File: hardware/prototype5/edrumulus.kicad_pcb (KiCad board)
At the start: 2 copper layers, 65 x 56.5 mm, 67 parts, among them J1 Trigger Connector, J2 Raspberry Pi GPIO pins, U1 ESP32-DEVKIT-V1

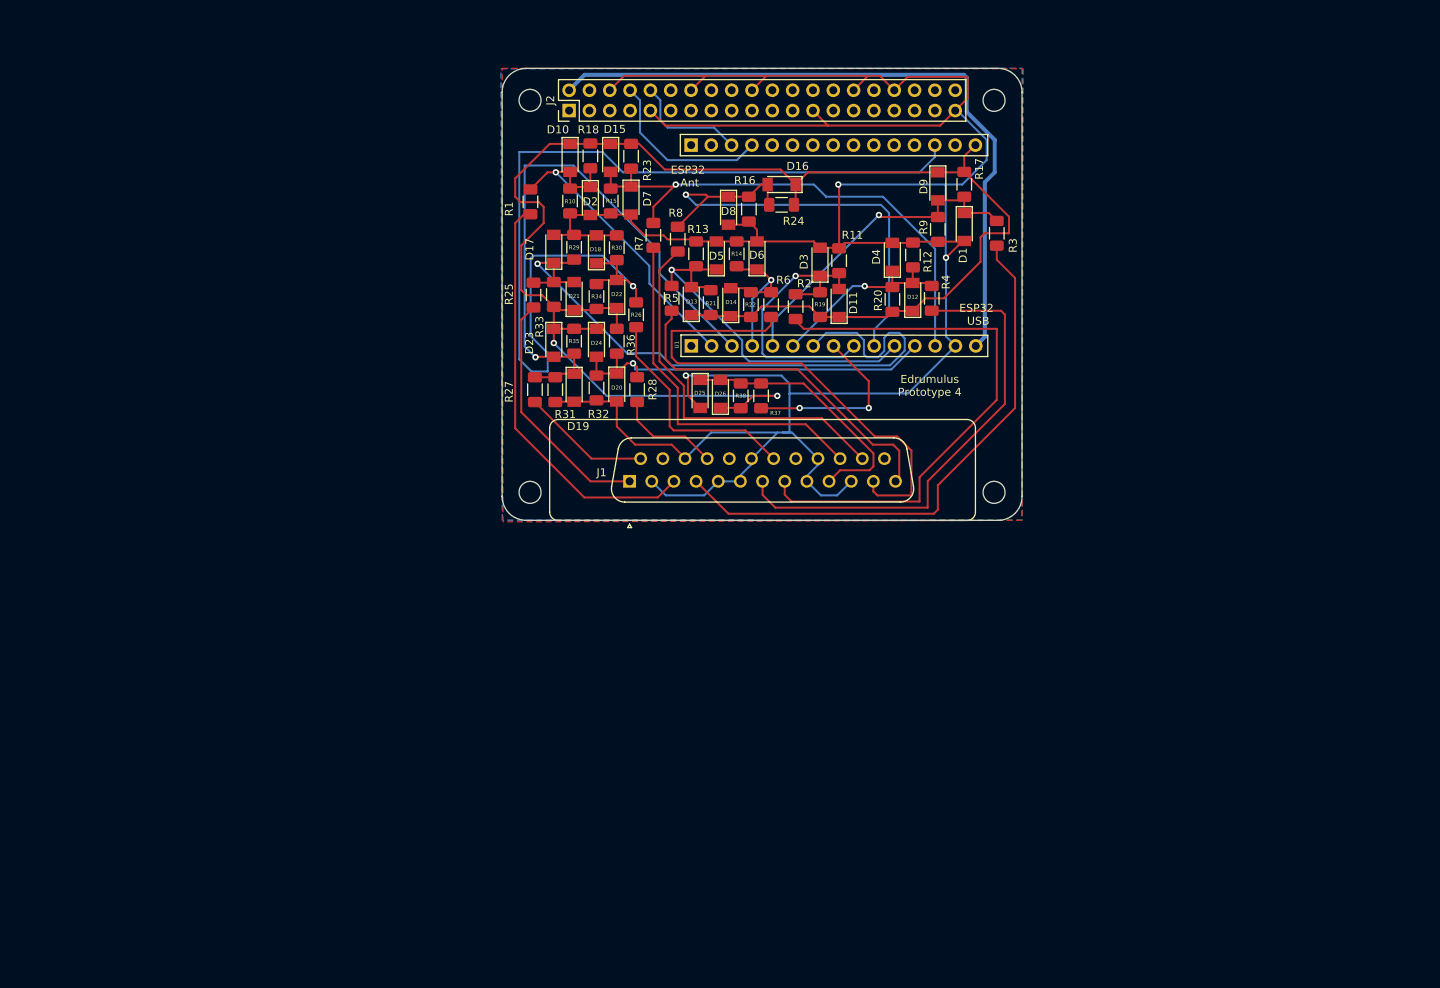
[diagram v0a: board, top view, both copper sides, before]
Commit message: some layout cleanup
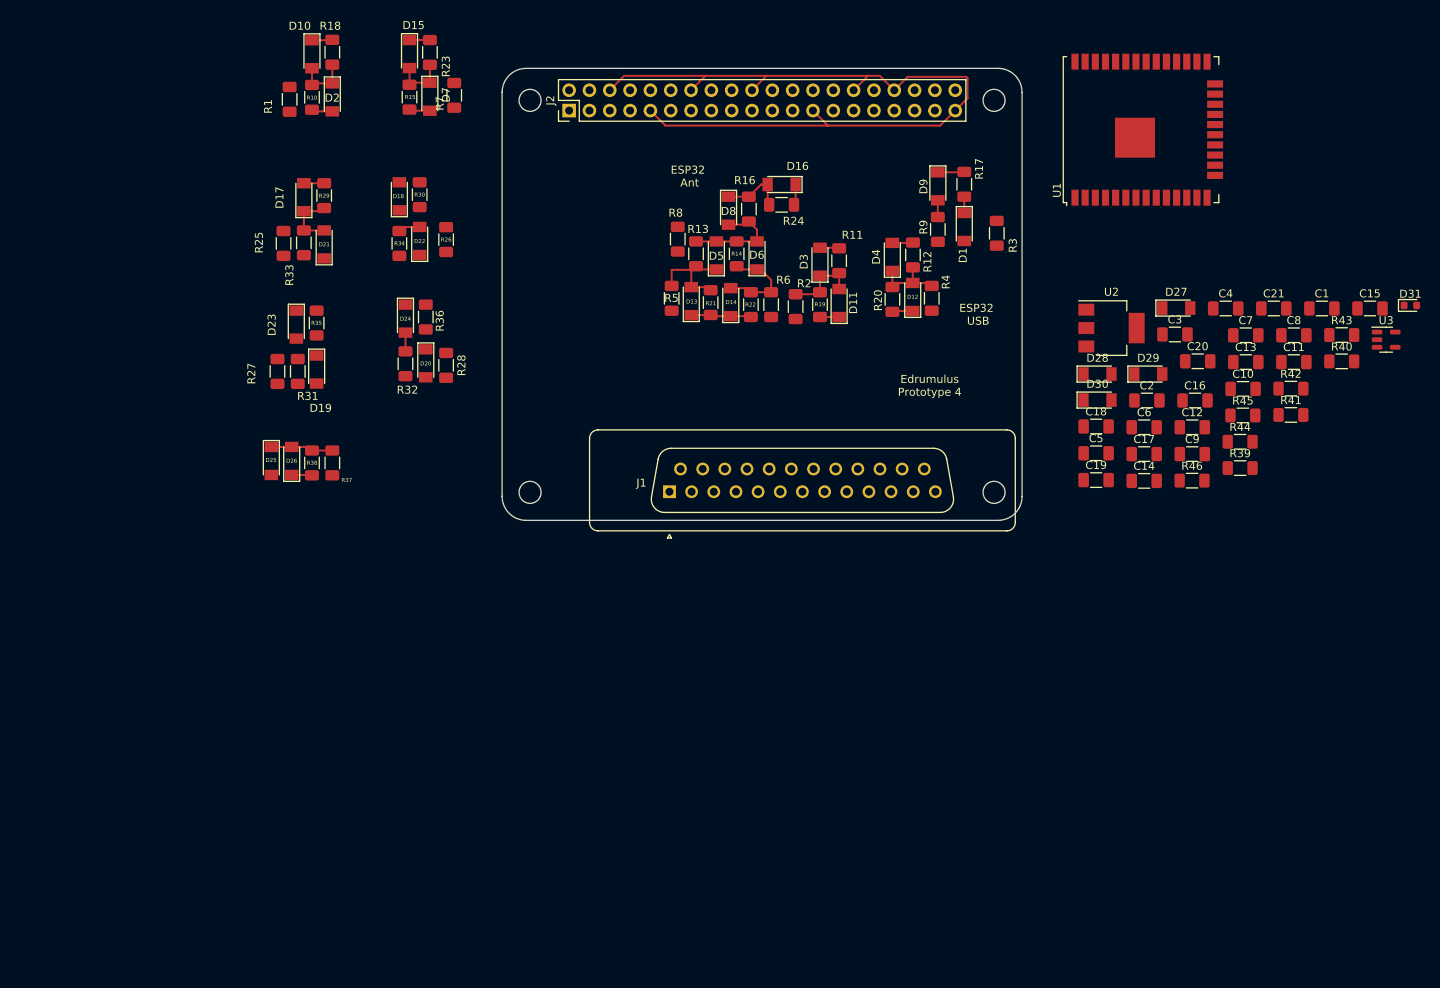
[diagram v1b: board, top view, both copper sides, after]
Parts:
- added C1: 100 nF, Capacitor_SMD:C_1206_3216Metric_Pad1.33x1.80mm_HandSolder, F.Cu at (209.0, 103.1)
- added C10: 100 nF, Capacitor_SMD:C_1206_3216Metric_Pad1.33x1.80mm_HandSolder, F.Cu at (199.2, 113.2)
- added C11: 100 nF, Capacitor_SMD:C_1206_3216Metric_Pad1.33x1.80mm_HandSolder, F.Cu at (205.5, 109.8)
- added C12: 100 nF, Capacitor_SMD:C_1206_3216Metric_Pad1.33x1.80mm_HandSolder, F.Cu at (192.8, 118.0)
- added C13: 100 nF, Capacitor_SMD:C_1206_3216Metric_Pad1.33x1.80mm_HandSolder, F.Cu at (199.5, 109.8)
- added C14: 100 nF, Capacitor_SMD:C_1206_3216Metric_Pad1.33x1.80mm_HandSolder, F.Cu at (186.8, 124.7)
- added C15: 100 nF, Capacitor_SMD:C_1206_3216Metric_Pad1.33x1.80mm_HandSolder, F.Cu at (215.1, 103.1)
- added C16: 1 µF, Capacitor_SMD:C_1206_3216Metric_Pad1.33x1.80mm_HandSolder, F.Cu at (193.2, 114.6)
- added C17: 22 µF, Capacitor_SMD:C_1206_3216Metric_Pad1.33x1.80mm_HandSolder, F.Cu at (186.8, 121.3)
- added C18: 10 nF, Capacitor_SMD:C_1206_3216Metric_Pad1.33x1.80mm_HandSolder, F.Cu at (180.8, 117.9)
- added C19: 10 µF, Capacitor_SMD:C_1206_3216Metric_Pad1.33x1.80mm_HandSolder, F.Cu at (180.8, 124.6)
- added C2: 100 nF, Capacitor_SMD:C_1206_3216Metric_Pad1.33x1.80mm_HandSolder, F.Cu at (187.2, 114.6)
- added C20: 1 µF, Capacitor_SMD:C_1206_3216Metric_Pad1.33x1.80mm_HandSolder, F.Cu at (193.5, 109.7)
- added C21: 22 µF, Capacitor_SMD:C_1206_3216Metric_Pad1.33x1.80mm_HandSolder, F.Cu at (203.0, 103.1)
- added C3: 100 nF, Capacitor_SMD:C_1206_3216Metric_Pad1.33x1.80mm_HandSolder, F.Cu at (190.7, 106.4)
- added C4: 100 nF, Capacitor_SMD:C_1206_3216Metric_Pad1.33x1.80mm_HandSolder, F.Cu at (197.0, 103.1)
- added C5: 100 nF, Capacitor_SMD:C_1206_3216Metric_Pad1.33x1.80mm_HandSolder, F.Cu at (180.8, 121.2)
- added C6: 100 nF, Capacitor_SMD:C_1206_3216Metric_Pad1.33x1.80mm_HandSolder, F.Cu at (186.8, 118.0)
- added C7: 100 nF, Capacitor_SMD:C_1206_3216Metric_Pad1.33x1.80mm_HandSolder, F.Cu at (199.5, 106.5)
- added C8: 100 nF, Capacitor_SMD:C_1206_3216Metric_Pad1.33x1.80mm_HandSolder, F.Cu at (205.5, 106.5)
- added C9: 100 nF, Capacitor_SMD:C_1206_3216Metric_Pad1.33x1.80mm_HandSolder, F.Cu at (192.8, 121.3)
- added D27: BAT85, Diode_SMD:D_MiniMELF, F.Cu at (190.8, 103.1)
- added D28: BAT85, Diode_SMD:D_MiniMELF, F.Cu at (181.0, 111.3)
- added D29: BAT85, Diode_SMD:D_MiniMELF, F.Cu at (187.3, 111.3)
- added D30: BAT85, Diode_SMD:D_MiniMELF, F.Cu at (181.0, 114.6)
- added D31: BOARD-LED, LED_SMD:LED_0603_1608Metric, F.Cu at (220.1, 102.7)
- added R39: 22 kOhm, Resistor_SMD:R_1206_3216Metric_Pad1.30x1.75mm_HandSolder, F.Cu at (198.8, 123.1)
- added R40: 22 kOhm, Resistor_SMD:R_1206_3216Metric_Pad1.30x1.75mm_HandSolder, F.Cu at (211.5, 109.7)
- added R41: 22 kOhm, Resistor_SMD:R_1206_3216Metric_Pad1.30x1.75mm_HandSolder, F.Cu at (205.2, 116.4)
- added R42: 22 kOhm, Resistor_SMD:R_1206_3216Metric_Pad1.30x1.75mm_HandSolder, F.Cu at (205.2, 113.1)
- added R43: 22 kOhm, Resistor_SMD:R_1206_3216Metric_Pad1.30x1.75mm_HandSolder, F.Cu at (211.5, 106.4)
- added R44: 22 kOhm, Resistor_SMD:R_1206_3216Metric_Pad1.30x1.75mm_HandSolder, F.Cu at (198.8, 119.8)
- added R45: 10 kOhm, Resistor_SMD:R_1206_3216Metric_Pad1.30x1.75mm_HandSolder, F.Cu at (199.2, 116.5)
- added R46: 470 Ohm, Resistor_SMD:R_1206_3216Metric_Pad1.30x1.75mm_HandSolder, F.Cu at (192.8, 124.6)
- added U2: AMS1117-3.3, Package_TO_SOT_SMD:SOT-223-3_TabPin2, F.Cu at (182.7, 105.6)
- added U3: LT1761-3.3, Package_TO_SOT_SMD:TSOT-23-5, F.Cu at (217.1, 107.0)
- R27, R28: value 100 kOhm -> 22 kOhm
- R30, R32, R35, R36: value 22 kOhm -> 100 kOhm
- U1: value ESP32-DEVKIT-V1 -> ESP32-WROOM-32U; footprint edrumulus:esp32_devkit_v1 -> RF_Module:ESP32-WROOM-32U
- moved U1 62.4 mm to (186.4, 80.8)
- moved D25 54.2 mm to (77.7, 122.2)
- moved D26 54.2 mm to (80.3, 122.2)
- moved R37 54.2 mm to (85.3, 122.4)
- moved R38 54.2 mm to (82.8, 122.4)
- moved R18 34.8 mm to (85.3, 71.1)
- moved D2 34.8 mm to (85.3, 76.7)
- moved R10 34.8 mm to (82.8, 76.7)
- moved D10 34.8 mm to (82.8, 71.3)
- moved R1 32.7 mm to (80.0, 77.0)
- moved D19 32.3 mm to (83.4, 110.8)
- moved D23 32.3 mm to (80.8, 105.1)
- moved R27 32.3 mm to (78.5, 111.0)
- moved R31 32.3 mm to (81.0, 111.0)
- moved R35 32.3 mm to (83.4, 104.9)
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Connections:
- D18 pad 1: GPIO15 -> GPIO2
- D19 pad 1: GPIO39 -> 3V3
- D19 pad 2: CRASH1-SLEEVE -> GPIO2
- D22 pad 1: 3V3 -> GPIO15
- D22 pad 2: GPIO15 -> CRASH1-SLEEVE
- D23 pad 2: GPIO39 -> GPIO12
- D24 pad 2: GPIO12 -> GPIO15
- J1 pad 15: unconnected-(J1-Pad15) -> TOM1-RING
- J1 pad 25: unconnected-(J1-Pad25) -> RIDE-BELL-TIP
- J2 pad 2: ESP-VIN -> RASPI-VIN
- R25 pad 1: KICK-TIP -> GPIO33
- R25 pad 2: GPIO33 -> KICK-TIP
- R26 pad 1: TOM3-TIP -> RIDE-BELL-TIP
- R26 pad 2: GPIO15 -> GPIO2
- R27 pad 1: TOM1-TIP -> GPIO2
- R27 pad 2: GPIO39 -> CRASH1-SLEEVE
- R28 pad 1: TOM2-TIP -> 3V3
- R28 pad 2: GPIO12 -> GPIO2
- R30 pad 1: GPIO15 -> GPIO12
- R30 pad 2: CRASH1-SLEEVE -> TOM2-TIP
- R31 pad 1: GPIO39 -> GPIO12
- R32 pad 1: GPIO12 -> GPIO15
- R32 pad 2: CRASH1-SLEEVE -> TOM3-TIP
- R34 pad 1: 3V3 -> GPIO15
- R34 pad 2: GPIO15 -> CRASH1-SLEEVE
- R35 pad 1: 3V3 -> TOM1-RING
- R35 pad 2: GPIO39 -> GPIO4
- R36 pad 1: 3V3 -> TOM1-TIP
- R36 pad 2: GPIO12 -> GPIO39
- U1 pad 1: unconnected-(U1-Pad1) -> CRASH1-SLEEVE
- U1 pad 10: GPIO27 -> GPIO25
- U1 pad 11: GPIO14 -> GPIO26
- U1 pad 12: GPIO12 -> GPIO27
- U1 pad 13: GPIO13 -> GPIO14
- U1 pad 14: CRASH1-SLEEVE -> GPIO12
- U1 pad 15: ESP-VIN -> CRASH1-SLEEVE
- U1 pad 16: 3V3 -> GPIO13
- U1 pad 17: CRASH1-SLEEVE -> unconnected-(U1-Pad17)
- U1 pad 18: GPIO15 -> unconnected-(U1-Pad18)
- U1 pad 2: GPIO36 -> ESP32-3V3
- U1 pad 23: unconnected-(U1-Pad23) -> GPIO15
- U1 pad 24: unconnected-(U1-Pad24) -> GPIO2
- U1 pad 26: unconnected-(U1-Pad26) -> GPIO4
- U1 pad 27: ESP-UART0-RX -> unconnected-(U1-Pad27)
- U1 pad 28: ESP-UART0-TX -> unconnected-(U1-Pad28)
- U1 pad 29: unconnected-(U1-Pad29) -> Net-(R46-Pad1)
- U1 pad 3: GPIO39 -> Net-(C20-Pad1)
- U1 pad 4: GPIO34 -> GPIO36
- U1 pad 5: GPIO35 -> GPIO39
- U1 pad 6: GPIO32 -> GPIO34
- U1 pad 7: GPIO33 -> GPIO35
- U1 pad 8: GPIO25 -> GPIO32
- U1 pad 9: GPIO26 -> GPIO33
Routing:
- net CRASH1-SLEEVE: track 350.1 -> 130.4 mm, vias 3 -> 0
- net 3V3: track 206.6 -> 26.2 mm, vias 2 -> 0
- net GPIO15: track 127.4 -> 2.34 mm, vias 1 -> 0
- net ESP-VIN: track 86.6 -> 0.00 mm
- net GPIO33: track 82.9 -> 7.83 mm, vias 1 -> 0
- net GPIO39: track 74.0 -> 0.00 mm, vias 1 -> 0
- net HI-HAT-RING: track 70.2 -> 0.00 mm
- net SNARE-RING: track 70.0 -> 0.00 mm
- net CRASH1-TIP: track 63.3 -> 0.00 mm
- net HI-HAT-TIP: track 60.5 -> 0.00 mm
- net GPIO13: track 66.5 -> 6.98 mm, vias 1 -> 0
- net GPIO27: track 62.6 -> 8.14 mm, vias 1 -> 0
- net SNARE-TIP: track 52.3 -> 0.00 mm
- net GPIO12: track 49.0 -> 0.00 mm, vias 1 -> 0
- net RIDE-TIP: track 47.4 -> 0.00 mm
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- removed copper zone on B.Cu, net CRASH1-SLEEVE
- removed copper zone on F.Cu, net CRASH1-SLEEVE

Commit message: some more prototype 5 development
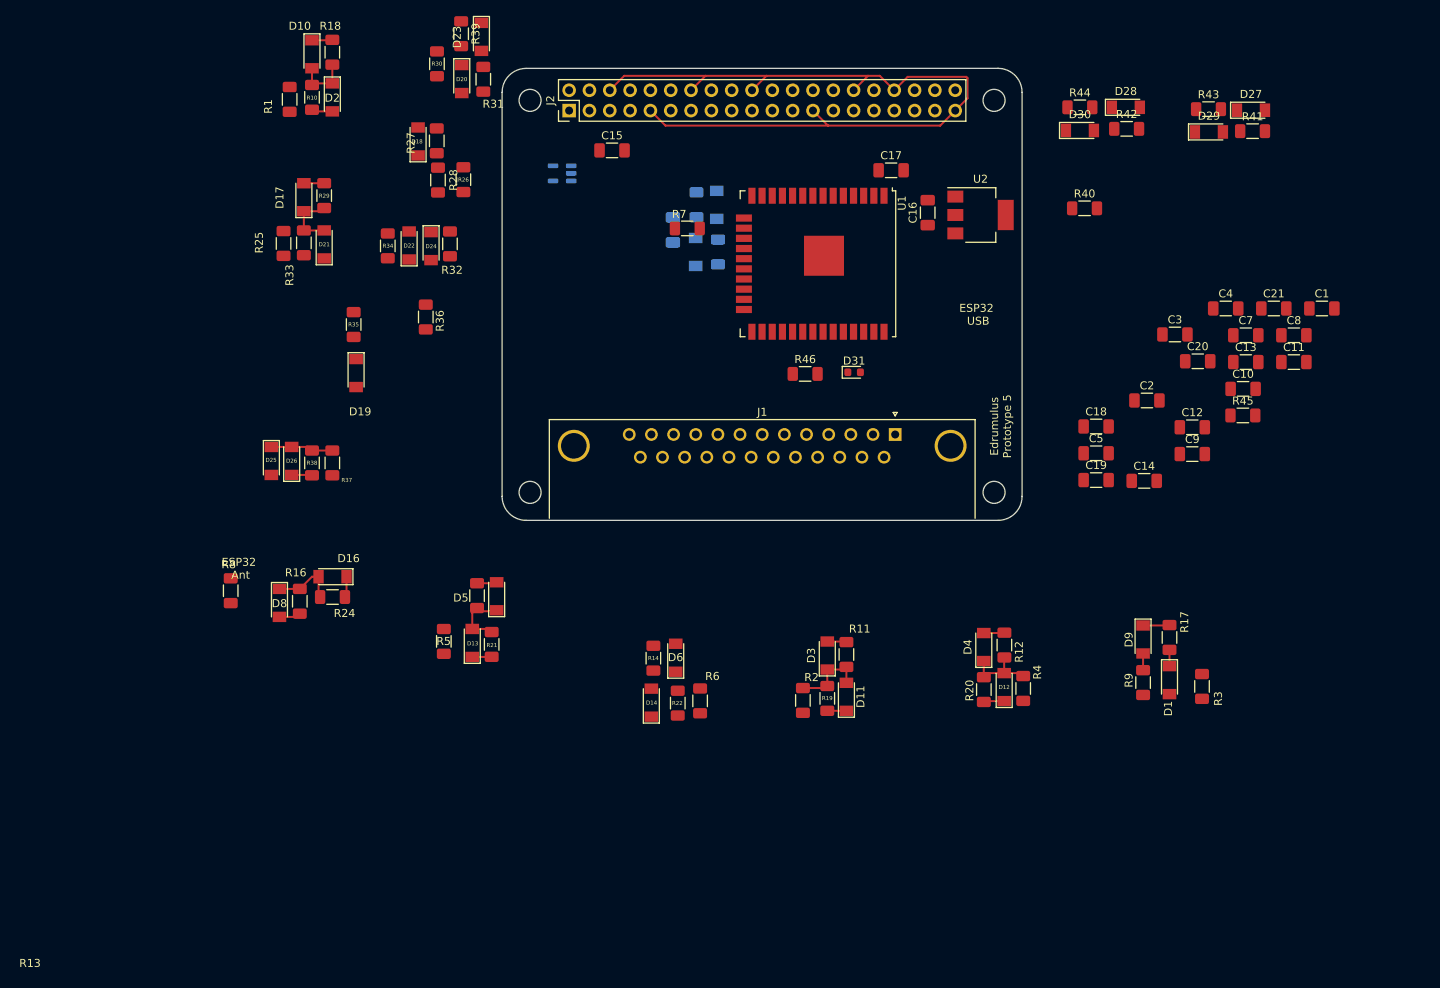
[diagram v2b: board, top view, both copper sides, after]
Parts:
- C6, D15, D7, R15, R23, U3: moved to B.Cu
- J1: footprint Connector_Dsub:DSUB-25_Female_Vertical_P2.77x2.84mm -> Connector_Dsub:DSUB-25_Female_Horizontal_P2.77x2.84mm_EdgePinOffset7.70mm_Housed_MountingHolesOffset9.12mm
- moved R39 111.5 mm to (101.4, 68.8), turned to -90 degrees
- moved U3 105.1 mm to (114.1, 86.2), turned to 180 degrees
- moved C15 96.8 mm to (120.3, 83.4)
- moved D16 74.5 mm to (85.4, 136.7)
- moved D8 74.5 mm to (78.7, 139.9)
- moved R16 74.5 mm to (81.3, 139.7)
- moved R24 74.5 mm to (85.4, 139.2)
- moved R8 71.1 mm to (72.6, 138.4)
- moved D31 70.0 mm to (150.6, 111.1)
- moved C6 63.9 mm to (127.9, 93.3), turned to 90 degrees
- moved R17 62.2 mm to (190.0, 144.2)
- moved D1 62.2 mm to (190.0, 149.6)
- moved D9 62.2 mm to (186.7, 144.5)
- moved R3 62.2 mm to (194.1, 150.4)
- moved R9 62.2 mm to (186.7, 149.9)
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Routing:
- net CRASH1-SLEEVE: track 130.4 -> 117.0 mm
- net GPIO34: track 11.8 -> 0.00 mm
- net 3V3: track 26.2 -> 18.5 mm
- net GPIO13: track 6.98 -> 0.00 mm
- net GPIO14: track 12.7 -> 8.15 mm
- net GPIO15: track 2.34 -> 0.00 mm
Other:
- board text added: "Edrumulus Prototype 5"
- board text removed: "Edrumulus Prototype 4"
